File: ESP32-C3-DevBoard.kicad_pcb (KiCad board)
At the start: 2 copper layers, 25.4 x 26 mm, 21 parts, among them J1 USB_C_Receptacle_USB2.0, J2 Conn_01x10, J3 Conn_01x10, SW1 SW_Push, SW2 SW_Push, U1 ESP32-C3-WROOM-02, U3 RT9080-33GJ5

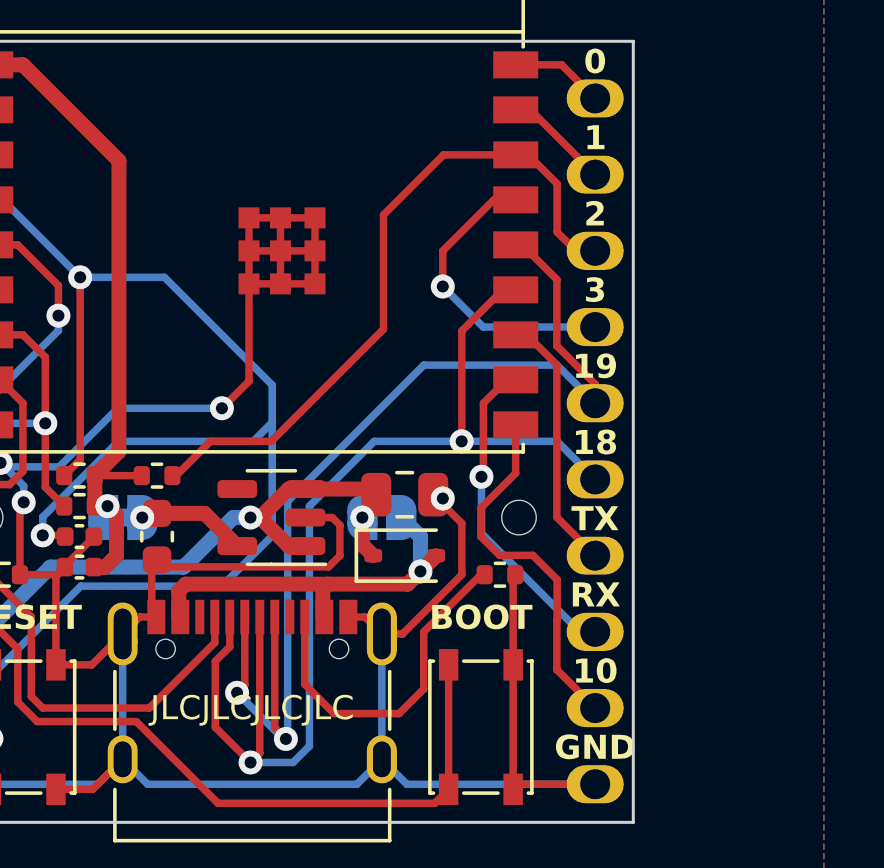
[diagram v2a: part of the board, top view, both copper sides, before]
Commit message: Add files via upload
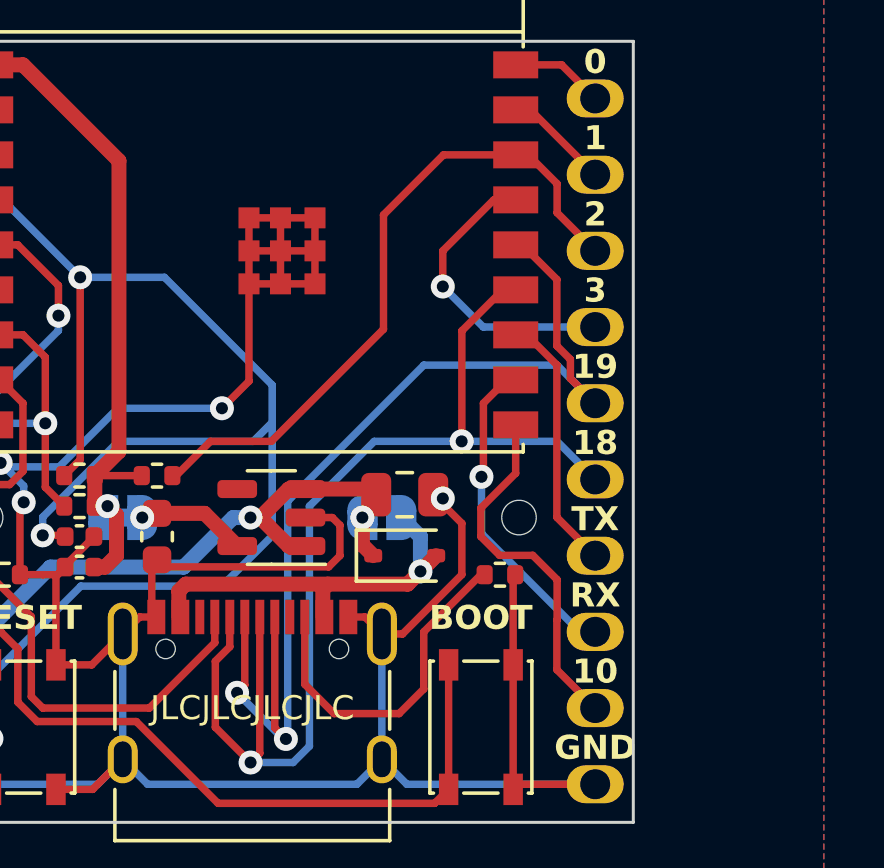
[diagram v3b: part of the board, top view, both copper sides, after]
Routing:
- net Net-(J1-CC2): track 11.0 -> 11.7 mm

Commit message: Add files via upload
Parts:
- C3: value 100nF -> 1uF
- C4: value 100nF -> 0.1uF
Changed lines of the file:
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@@
         (effects (font (size 1 1) (thickness 0.15)))
     )
-    (fp_text value "100nF" (at 0 1.16) (layer "F.Fab")
+    (fp_text value "0.1uF" (at 0 1.16) (layer "F.Fab")
         (effects (font (size 1 1) (thickness 0.15)))
     )
@@
     (descr "Capacitor SMD 0402 (1005 Metric), square (rectangular) end terminal, IPC_7351 nominal, (Body size source: IPC-SM-782 page 76, https://www.pcb-3d.com/wordpress/wp-content/uploads/ipc-sm-782a_amendment_1_and_2.pdf), generated with kicad-footprint-generator")
     (tags "capacitor")
-    (property "LCSC" "C1525")
+    (property "LCSC" "C52923")
     (property "Sheetfile" "ESP32-C3-DevBoard.kicad_sch")
     (property "Sheetname" "")
@@
         (effects (font (size 1 1) (thickness 0.15)))
     )
-    (fp_text value "100nF" (at 0 1.16) (layer "F.Fab")
-        (effects (font (size 1 1) (thickness 0.15)))
-    )
+    (fp_text value "1uF" (at 0 1.16) (layer "F.Fab")
+        (effects (font (size 1 1) (thickness 0.15)))
+    )
